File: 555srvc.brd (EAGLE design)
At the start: 31 x 30.5 mm, 12 parts, among them IC1 NE555D

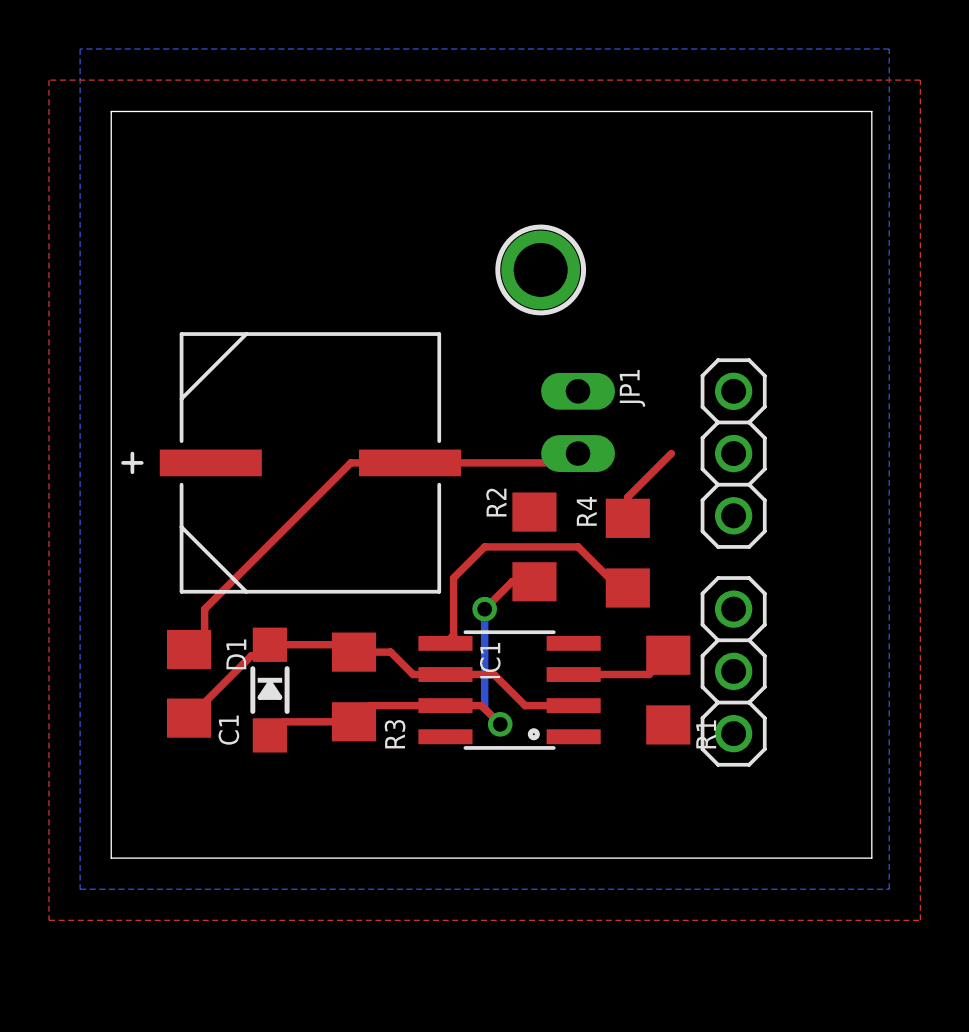
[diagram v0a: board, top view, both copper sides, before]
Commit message: smd added schema and board pdf,png
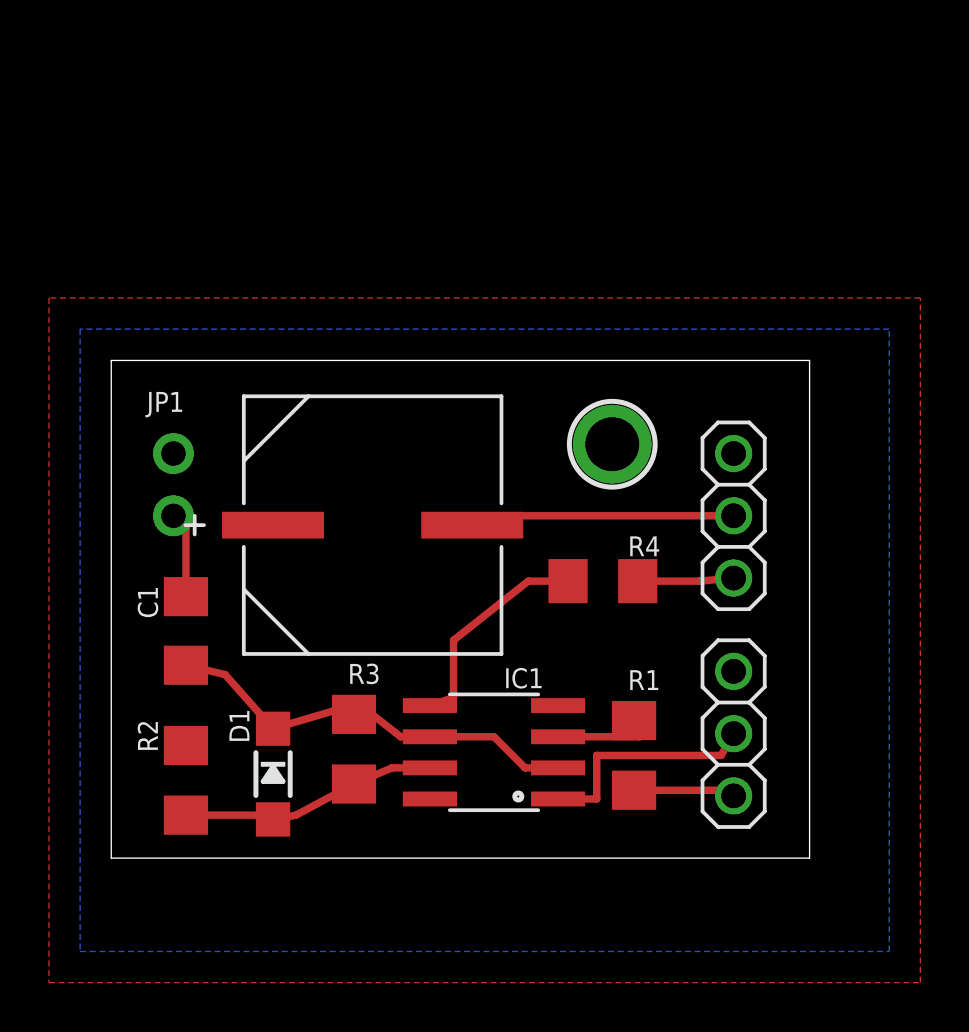
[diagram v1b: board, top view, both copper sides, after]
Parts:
- IC1: value NE555D -> 555
- JP1: device microbuilder:1X02_OVAL -> microbuilder:1X02_ROUND
- moved R2 17.1 mm to (3.05, 3.17)
- moved JP1 16.7 mm to (2.54, 15.2)
- moved U$6 7.69 mm to (20.4, 16.9)
- moved C2 3.59 mm to (10.7, 13.6)
- moved D1 3.43 mm to (6.60, 3.43)
- moved R1 3.01 mm to (21.3, 4.19)
- moved IC1 2.62 mm to (15.6, 4.32)
- moved JP3 2.54 mm to (25.4, 14.0)
- moved JP2 2.54 mm to (25.4, 5.08)
- moved R3 2.54 mm to (9.91, 4.45)
- moved C1 2.16 mm to (3.05, 9.27)
- moved R4 1.53 mm to (20.1, 11.3), turned to 0 degrees
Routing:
- net N$2: track 17.7 -> 10.5 mm, vias 2 -> 0
- net SERVO_OUT: track 0.00 -> 4.16 mm
- net N$4: track 11.1 -> 8.87 mm
- net GND: track 21.5 -> 23.7 mm
- net N$1: track 18.0 -> 17.3 mm
- net INPUT: track 3.38 -> 3.92 mm
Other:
- board size 31 x 30.5 mm -> 28.5 x 20.3 mm

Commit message: smd wip
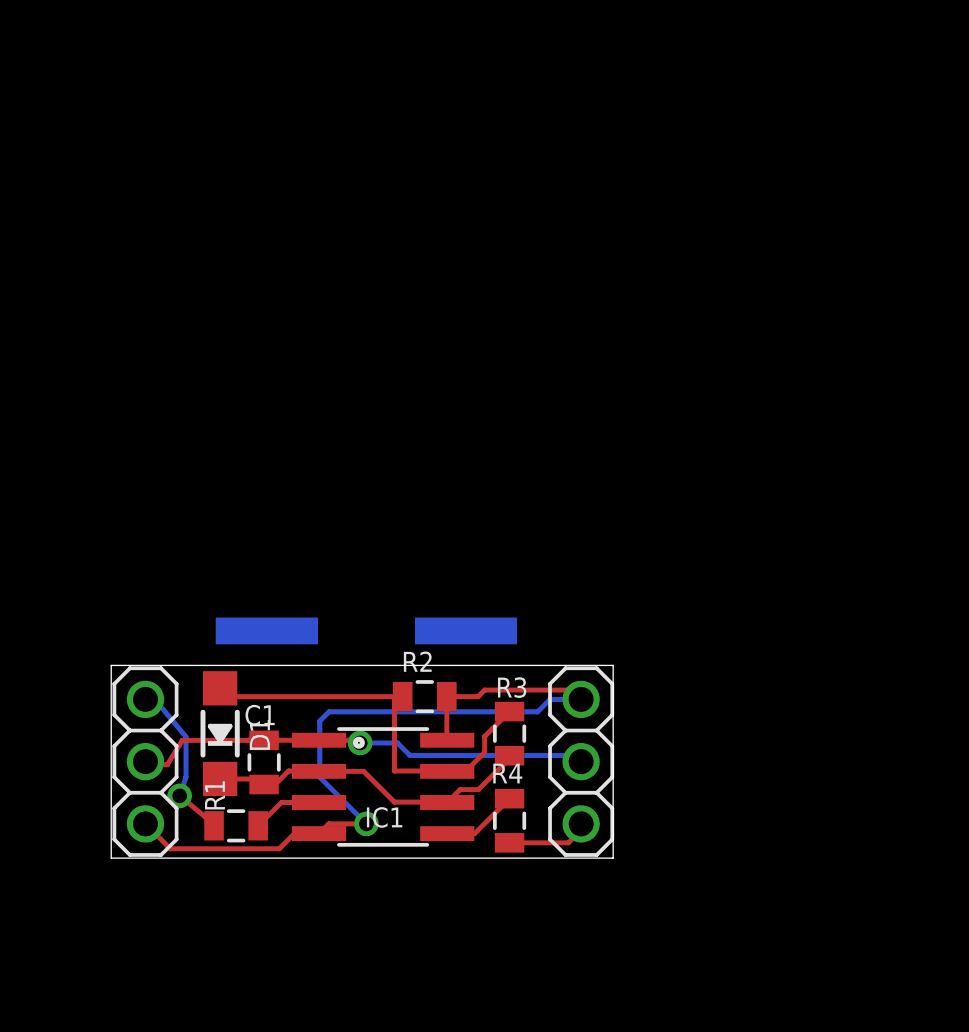
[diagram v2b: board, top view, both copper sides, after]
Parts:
- removed JP1: 4.5-5.5V, microbuilder:1X02_ROUND
- removed U$6: MOUNTINGHOLE2.0, microbuilder:MOUNTINGHOLE_2.0_PLATED
- C1: device SparkFun-Capacitors:1206 -> ATtami:0805
- R1, R2, R3, R4: device adafruit:R1206 -> ATtami:0805
- moved JP2 24.0 mm to (1.40, 3.94), turned to 90 degrees
- moved R1 16.5 mm to (5.10, 1.32), turned to 180 degrees
- moved JP3 11.8 mm to (19.2, 3.94)
- moved R4 10.5 mm to (16.3, 1.52), turned to 270 degrees
- moved R2 10.3 mm to (12.8, 6.59), turned to 180 degrees
- moved R3 6.38 mm to (16.3, 5.08), turned to 90 degrees
- moved C1 6.24 mm to (6.24, 3.90)
- moved IC1 4.74 mm to (11.1, 2.90), turned to 270 degrees
- moved C2 4.33 mm to (10.4, 9.27), flipped to the bottom, turned to 180 degrees
- moved D1 2.72 mm to (4.44, 5.08), turned to 90 degrees
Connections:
- net GND: no longer JP1.2
- net VCC: no longer JP1.1
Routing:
- net VCC: track 0.00 -> 33.4 mm, vias 0 -> 1
- net N$2: track 10.5 -> 18.8 mm
- net N$4: track 8.87 -> 3.13 mm
- net N$1: track 17.3 -> 13.6 mm
- net GND: track 23.7 -> 20.0 mm, vias 0 -> 1
- net SERVO_OUT: track 4.16 -> 6.68 mm, vias 0 -> 1
- net N$5: track 4.03 -> 2.88 mm
- net INPUT: track 3.92 -> 4.47 mm
- removed copper zone on layer 16, net GND
- removed copper zone on layer 1, net VCC
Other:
- board size 28.5 x 20.3 mm -> 20.5 x 7.9 mm

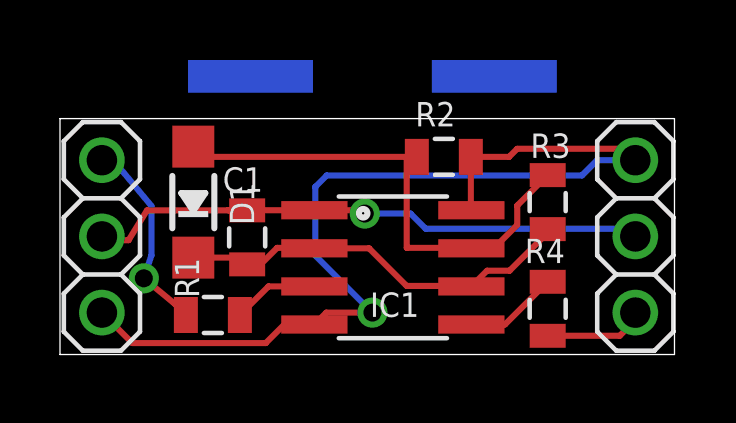
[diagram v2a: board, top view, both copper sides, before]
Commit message: board layout
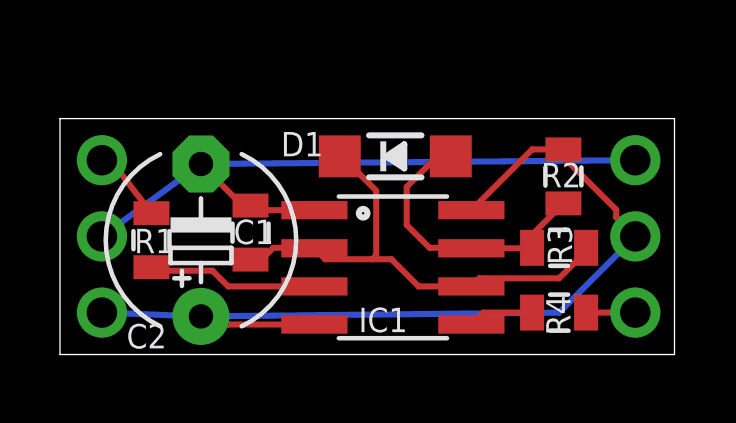
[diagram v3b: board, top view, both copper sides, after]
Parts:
- C2: value 1000UF -> (none); device Panasonic-EEE0_EEE1_EEE2_EEEFC:CAPAE1030X1050N -> adafruit:E5-6
- JP2, JP3: device adafruit:1X03 -> adafruit:1X03-CLEANBIG
- moved C2 7.90 mm to (4.70, 3.81), flipped to the top, turned to 90 degrees
- moved D1 6.90 mm to (11.2, 6.61), turned to 0 degrees
- moved R2 4.04 mm to (16.8, 5.94), turned to 270 degrees
- moved R1 3.23 mm to (3.05, 3.81), turned to 90 degrees
- moved R3 1.57 mm to (16.6, 3.56), turned to 180 degrees
- moved R4 0.40 mm to (16.6, 1.40), turned to 0 degrees
- moved C1 0.19 mm to (6.35, 4.06)
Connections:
- net GND: now also C2.-, JP3.1; no longer C2.2, JP3.2
- net VCC: now also C2.+, JP3.2; no longer C2.1, JP3.1
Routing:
- net N$2: track 18.8 -> 10.1 mm
- net SERVO_OUT: track 6.68 -> 2.52 mm, vias 1 -> 0
- net GND: track 20.0 -> 23.0 mm, vias 1 -> 0
- net VCC: track 33.4 -> 30.5 mm, vias 1 -> 0
- net N$1: track 13.6 -> 16.5 mm
- net INPUT: track 4.47 -> 1.64 mm
- net N$5: track 2.88 -> 5.70 mm
- net N$4: track 3.13 -> 2.19 mm
